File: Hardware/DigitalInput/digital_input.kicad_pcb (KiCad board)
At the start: 4 copper layers, 70 x 67.5 mm, 83 parts, among them J1 DIGITAL INPUT, J2 NUCLEO LEFT, J3 NUCLEO RIGHT, Q1 SI2347DS, Q2 SI2347DS, Q3 SI2347DS, Q4 SI2347DS, Q5 SI2347DS, Q6 SI2347DS, Q7 SI2347DS, Q8 SI2347DS, U1 VO615A-3, U2 VO615A-3, U3 VO615A-3, U4 VO615A-3, U5 VO615A-3, U6 VO615A-3, U7 VO615A-3, U8 VO615A-3

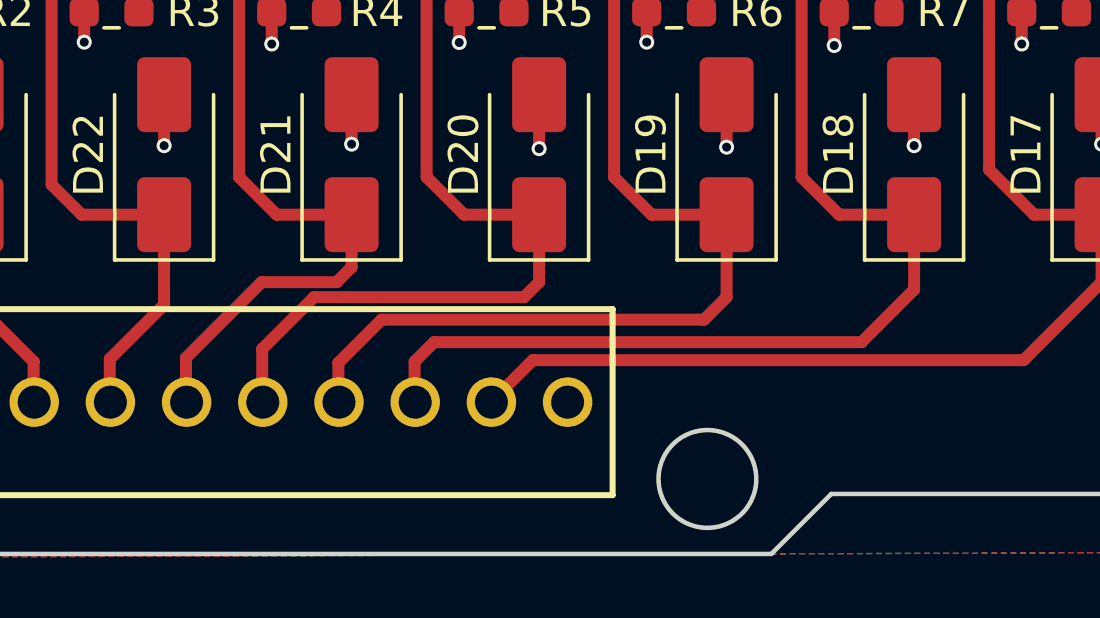
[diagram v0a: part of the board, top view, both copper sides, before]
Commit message: small adjustments and final revision
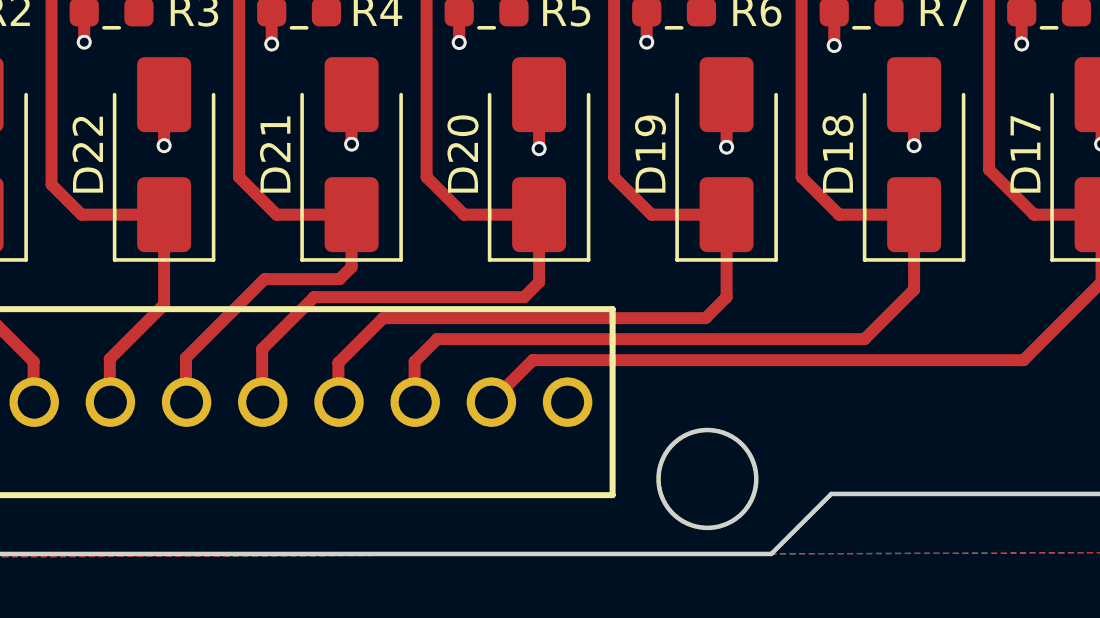
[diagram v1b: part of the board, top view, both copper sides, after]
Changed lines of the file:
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@@
 		(layer "Edge.Cuts")
+	)
+	(dimension
+		(type orthogonal)
+		(layer "Dwgs.User")
+		(pts
+			(xy 115.99 112.06) (xy 185.99 112.06)
+		)
+		(height 13.94)
+		(orientation 0)
+		(format
+			(prefix "")
+			(suffix "")
+			(units 3)
+			(units_format 1)
+			(precision 4)
+			(suppress_zeroes yes)
+		)
+		(style
+			(thickness 0.1)
+			(arrow_length 1.27)
+			(text_position_mode 1)
+			(arrow_direction outward)
+			(extension_height 0.58642)
+			(extension_offset 0.5)
+			(keep_text_aligned yes)
+		)
+		(gr_text "70 mm"
+			(at 150.99 126 0)
+			(layer "Dwgs.User")
+			(effects
+				(font
+					(size 0.8 0.8)
+					(thickness 0.1)
+				)
+			)
+		)
+	)
+	(dimension
+		(type orthogonal)
+		(layer "Dwgs.User")
+		(pts
+			(xy 161.99 116.06) (xy 166.99 48.56)
+		)
+		(height 34.01)
+		(orientation 1)
+		(format
+			(prefix "")
+			(suffix "")
+			(units 3)
+			(units_format 1)
+			(precision 4)
+			(suppress_zeroes yes)
+		)
+		(style
+			(thickness 0.1)
+			(arrow_length 1.27)
+			(text_position_mode 1)
+			(arrow_direction outward)
+			(extension_height 0.58642)
+			(extension_offset 0.5)
+			(keep_text_aligned yes)
+		)
+		(gr_text "67.5 mm"
+			(at 196 82.31 90)
+			(layer "Dwgs.User")
+			(effects
+				(font
+					(size 0.8 0.8)
+					(thickness 0.1)
+				)
+			)
+		)
+	)
+	(dimension
+		(type orthogonal)
+		(layer "Dwgs.User")
+		(pts
+			(xy 118.03 51.205) (xy 183.98 51.205)
+		)
+		(height -5.205)
+		(orientation 0)
+		(format
+			(prefix "")
+			(suffix "")
+			(units 3)
+			(units_format 1)
+			(precision 4)
+			(suppress_zeroes yes)
+		)
+		(style
+			(thickness 0.1)
+			(arrow_length 1.27)
+			(text_position_mode 1)
+			(arrow_direction outward)
+			(extension_height 0.58642)
+			(extension_offset 0.5)
+			(keep_text_aligned yes)
+		)
+		(gr_text "65.95 mm"
+			(at 151.005 46 0)
+			(layer "Dwgs.User")
+			(effects
+				(font
+					(size 0.8 0.8)
+					(thickness 0.1)
+				)
+			)
+		)
 	)
 	(segment
@@
 	)
 	(segment
+		(start 166.75 107.25)
+		(end 166.75 104.75)
+		(width 0.4)
+		(layer "F.Cu")
+		(net 56)
+	)
+	(segment
+		(start 165.1 108.9)
+		(end 166.75 107.25)
+		(width 0.4)
+		(layer "F.Cu")
+		(net 56)
+	)
+	(segment
 		(start 164 96.5)
 		(end 164 95.55)
@@
 	)
 	(segment
+		(start 150.85 108.9)
+		(end 165.1 108.9)
+		(width 0.4)
+		(layer "F.Cu")
+		(net 56)
+	)
+	(segment
+		(start 150.1 111)
+		(end 150.1 109.65)
+		(width 0.4)
+		(layer "F.Cu")
+		(net 56)
+	)
+	(segment
 		(start 164.25 104.75)
 		(end 163 103.5)
@@
 	)
 	(segment
-		(start 150.1 111)
-		(end 150.1 109.65)
-		(width 0.4)
-		(layer "F.Cu")
-		(net 56)
-	)
-	(segment
-		(start 166.75 107.25)
-		(end 166.75 104.75)
-		(width 0.4)
-		(layer "F.Cu")
-		(net 56)
-	)
-	(segment
 		(start 163 97.5)
 		(end 164 96.5)
@@
 	(segment
 		(start 150.1 109.65)
-		(end 150.75 109)
+		(end 150.85 108.9)
 		(width 0.4)
 		(layer "F.Cu")
 		(net 56)
-	)
-	(segment
-		(start 165 109)
-		(end 166.75 107.25)
-		(width 0.4)
-		(layer "F.Cu")
-		(net 56)
-	)
-	(segment
-		(start 150.75 109)
-		(end 165 109)
-		(width 0.4)
-		(layer "F.Cu")
-		(net 56)
-	)
-	(segment
-		(start 147.56 109.69)
-		(end 149 108.25)
-		(width 0.4)
-		(layer "F.Cu")
-		(net 57)
 	)
 	(segment
@@
 	)
 	(segment
-		(start 149 108.25)
-		(end 159.75 108.25)
+		(start 160.5 107.5)
+		(end 160.5 104.75)
+		(width 0.4)
+		(layer "F.Cu")
+		(net 57)
+	)
+	(segment
+		(start 149.05 108.2)
+		(end 159.8 108.2)
+		(width 0.4)
+		(layer "F.Cu")
+		(net 57)
+	)
+	(segment
+		(start 159.8 108.2)
+		(end 160.5 107.5)
+		(width 0.4)
+		(layer "F.Cu")
+		(net 57)
+	)
+	(segment
+		(start 147.56 109.69)
+		(end 149.05 108.2)
 		(width 0.4)
 		(layer "F.Cu")
@@
 	)
 	(segment
-		(start 160.5 107.5)
-		(end 160.5 104.75)
-		(width 0.4)
-		(layer "F.Cu")
-		(net 57)
-	)
-	(segment
 		(start 157.75 96.5)
 		(end 156.75 97.5)
@@
 	)
 	(segment
-		(start 159.75 108.25)
-		(end 160.5 107.5)
-		(width 0.4)
-		(layer "F.Cu")
-		(net 57)
-	)
-	(segment
 		(start 156.75 97.5)
 		(end 156.75 103.5)
@@
 	)
 	(segment
-		(start 148 106.5)
-		(end 147.5 107)
+		(start 147.6 106.9)
+		(end 145.1 106.9)
 		(width 0.4)
 		(layer "F.Cu")
@@
 	)
 	(segment
+		(start 148 106.5)
+		(end 147.6 106.9)
+		(width 0.4)
+		(layer "F.Cu")
+		(net 59)
+	)
+	(segment
 		(start 142.48 109.52)
 		(end 142.48 111)
@@
 	)
 	(segment
+		(start 145.1 106.9)
+		(end 142.48 109.52)
+		(width 0.4)
+		(layer "F.Cu")
+		(net 59)
+	)
+	(segment
 		(start 144.25 103.5)
 		(end 145.5 104.75)
@@
 	)
 	(segment
-		(start 147.5 107)
-		(end 145 107)
-		(width 0.4)
-		(layer "F.Cu")
-		(net 59)
-	)
-	(segment
 		(start 145.5 104.75)
 		(end 148 104.75)
 		(width 0.4)
 		(layer "F.Cu")
-		(net 59)
-	)
-	(segment
-		(start 145 107)
-		(end 142.48 109.52)
-		(width 0.4)
-		(layer "F.Cu")
